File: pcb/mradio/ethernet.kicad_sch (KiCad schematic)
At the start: 28 parts, among them J301 JX0026D21BNL, U301 DP83825I, Y301 DSC1525JL2A-25M00000T

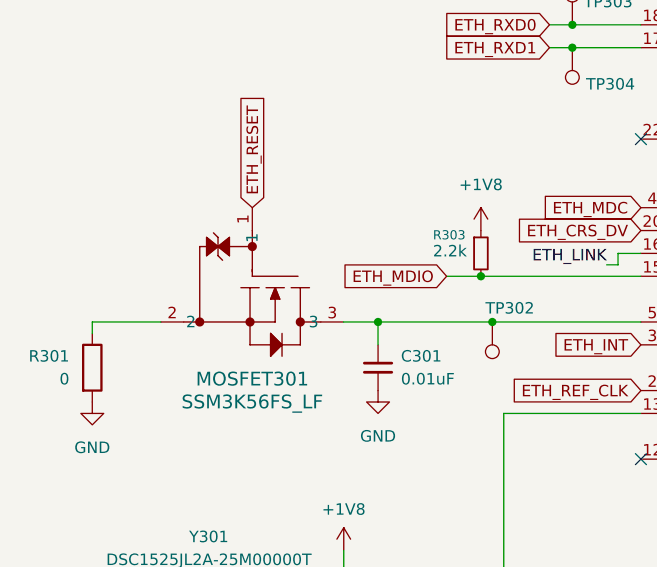
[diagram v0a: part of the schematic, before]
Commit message: library change
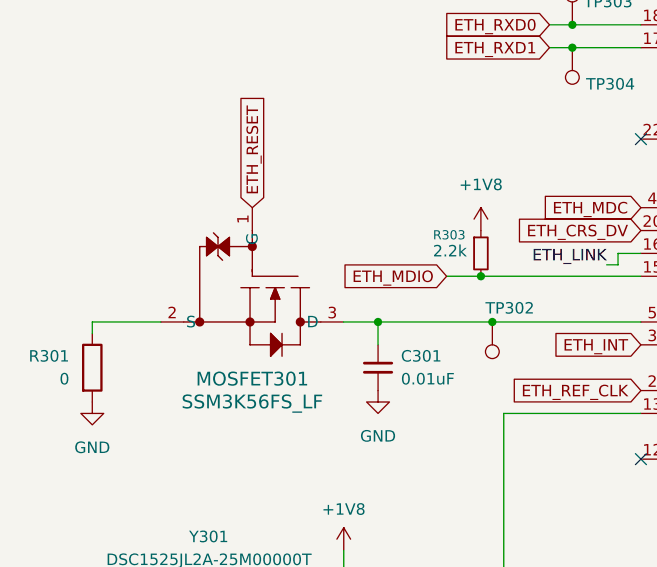
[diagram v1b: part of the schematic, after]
